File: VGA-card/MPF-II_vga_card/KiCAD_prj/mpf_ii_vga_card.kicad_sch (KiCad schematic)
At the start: 5 parts, among them J1 AppleBus, U1 74LVC245, U2 74LVC245, U3 74LVC245, U4 74LVC245

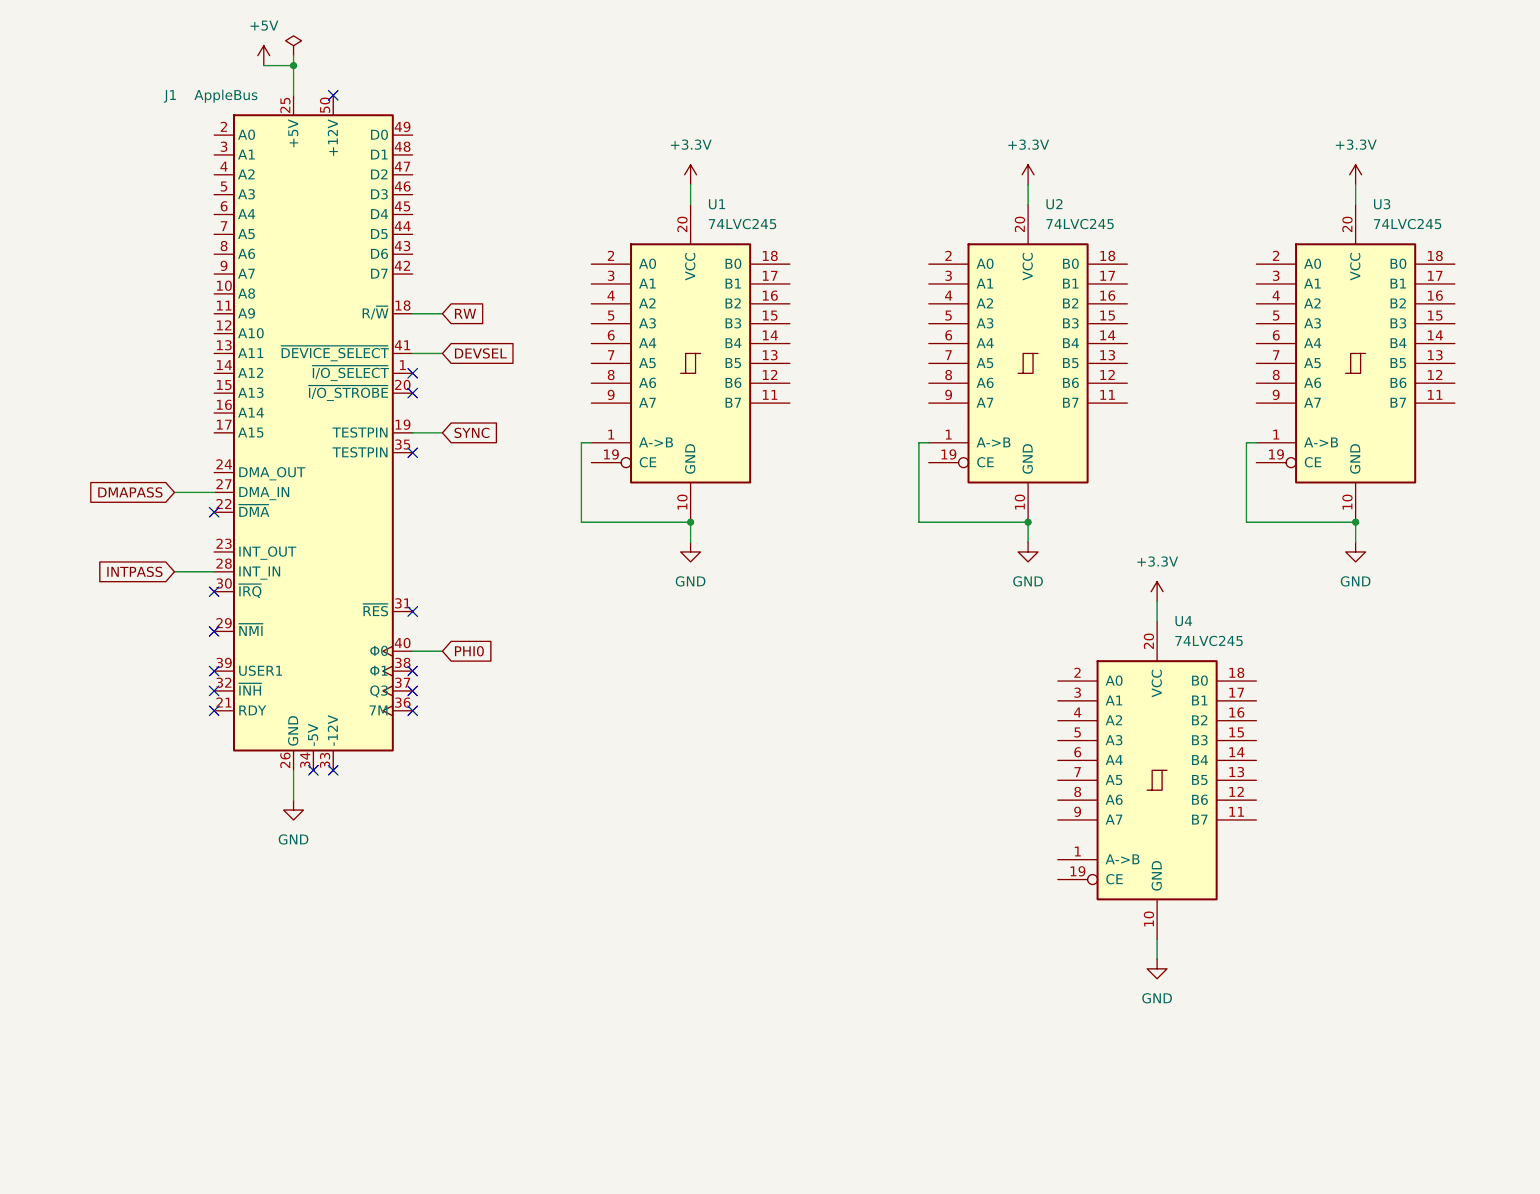
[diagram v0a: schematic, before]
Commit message: Schematics updated
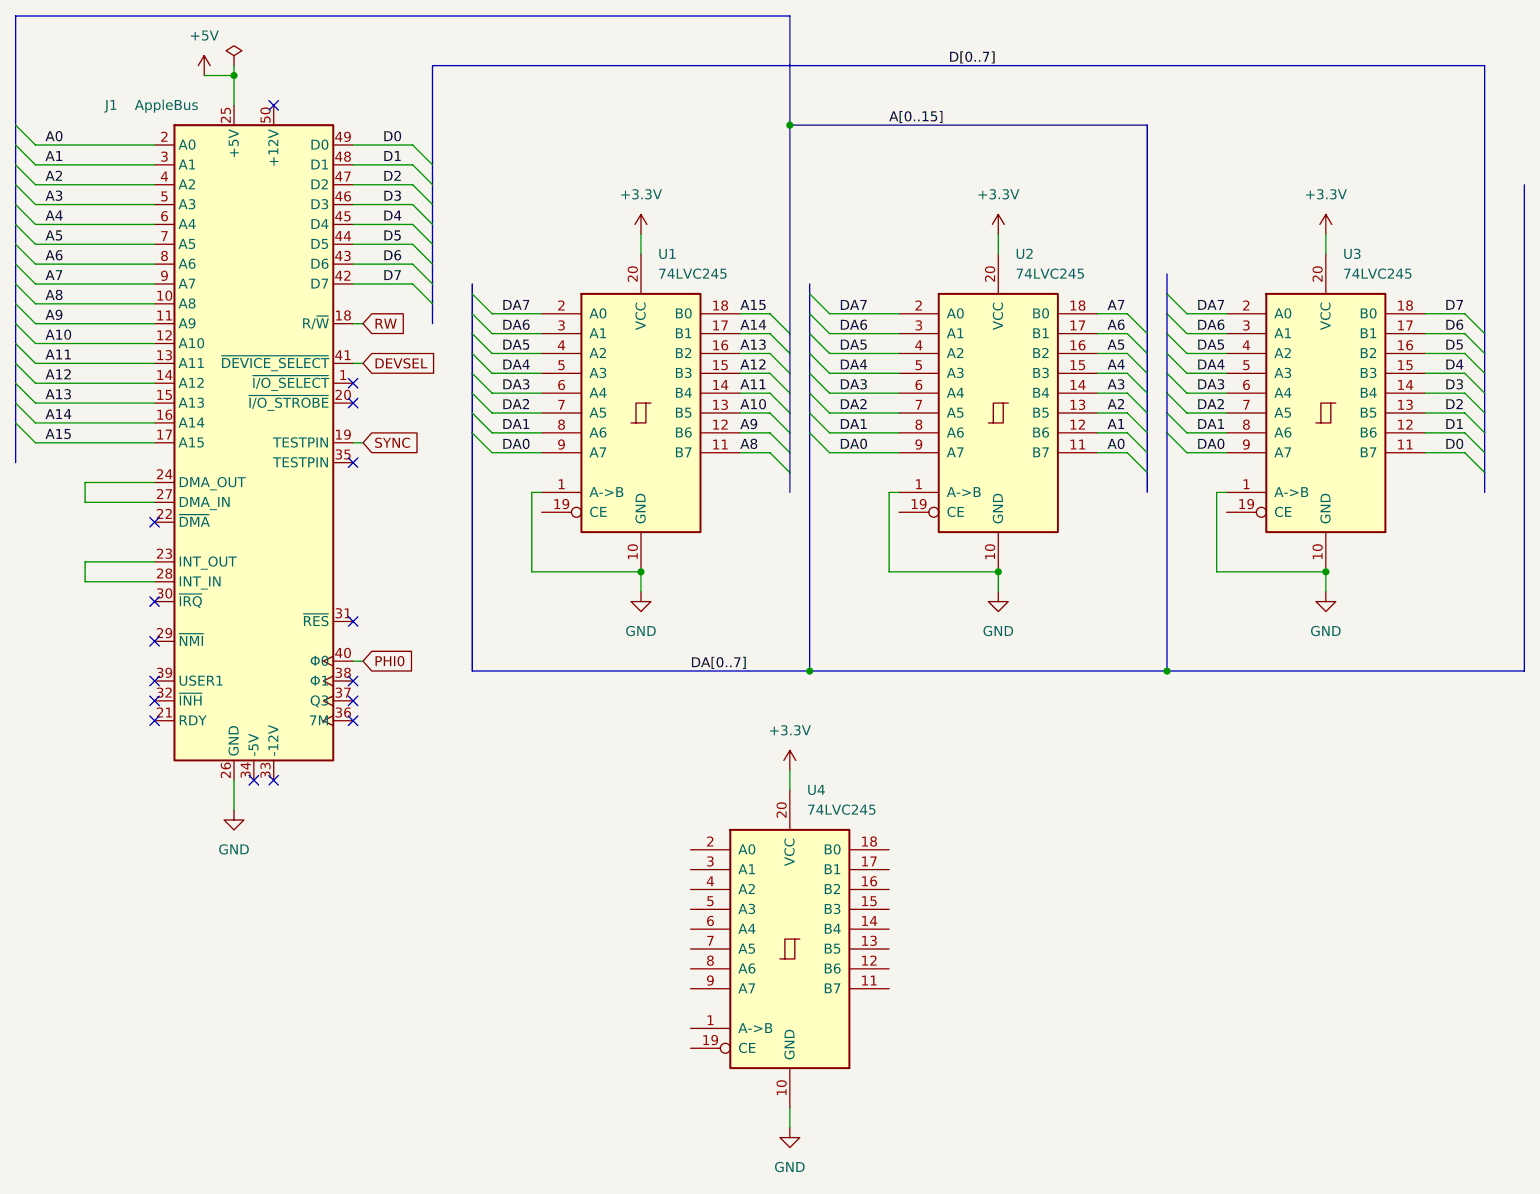
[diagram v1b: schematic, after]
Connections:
- net DMAPASS is gone; now on an unnamed net: J1.27 (DMA_IN)
- net INTPASS is gone; now on an unnamed net: J1.28 (INT_IN)
- net A8: now reaches J1.10 (A8)
- net A8: now also U1.11 (B7)
- net A9: now reaches J1.11 (A9)
- net A9: now also U1.12 (B6)
- net A10: now reaches J1.12 (A10)
- net A10: now also U1.13 (B5)
- net A11: now reaches J1.13 (A11)
- net A11: now also U1.14 (B4)
- net A12: now reaches J1.14 (A12)
- net A12: now also U1.15 (B3)
- net A13: now reaches J1.15 (A13)
- net A13: now also U1.16 (B2)
- net A14: now reaches J1.16 (A14)
- net A14: now also U1.17 (B1)
- net A15: now reaches J1.17 (A15)
- net A15: now also U1.18 (B0)
- net A0: now reaches J1.2 (A0)
- net A0: now also U2.11 (B7)
- net A1: now reaches J1.3 (A1)
- net A1: now also U2.12 (B6)
- net A2: now reaches J1.4 (A2)
- net A2: now also U2.13 (B5)
- net D7: now reaches J1.42 (D7)
- net D7: now also U3.18 (B0)
- net D6: now reaches J1.43 (D6)
- net D6: now also U3.17 (B1)
- net D5: now reaches J1.44 (D5)
- net D5: now also U3.16 (B2)
- net D4: now reaches J1.45 (D4)
- net D4: now also U3.15 (B3)
- net D3: now reaches J1.46 (D3)
- net D3: now also U3.14 (B4)
- net D2: now reaches J1.47 (D2)
- net D2: now also U3.13 (B5)
- net D1: now reaches J1.48 (D1)
- net D1: now also U3.12 (B6)
- net D0: now reaches J1.49 (D0)
- net D0: now also U3.11 (B7)
- net A3: now reaches J1.5 (A3)
- net A3: now also U2.14 (B4)
- net A4: now reaches J1.6 (A4)
- net A4: now also U2.15 (B3)
- net A5: now reaches J1.7 (A5)
- net A5: now also U2.16 (B2)
- net A6: now reaches J1.8 (A6)
- net A6: now also U2.17 (B1)
- net A7: now reaches J1.9 (A7)
- net A7: now also U2.18 (B0)
- net DA7: now reaches U3.2 (A0)
- net DA7: now also U1.2 (A0), U2.2 (A0)
- net DA6: now reaches U3.3 (A1)
- net DA6: now also U1.3 (A1), U2.3 (A1)
- net DA5: now reaches U3.4 (A2)
- net DA5: now also U1.4 (A2), U2.4 (A2)
- net DA4: now reaches U3.5 (A3)
- net DA4: now also U1.5 (A3), U2.5 (A3)
- net DA3: now reaches U3.6 (A4)
- net DA3: now also U1.6 (A4), U2.6 (A4)
- net DA2: now reaches U3.7 (A5)
- net DA2: now also U1.7 (A5), U2.7 (A5)
- net DA1: now reaches U3.8 (A6)
- net DA1: now also U1.8 (A6), U2.8 (A6)
- net DA0: now reaches U3.9 (A7)
- net DA0: now also U1.9 (A7), U2.9 (A7)
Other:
- moved on the sheet: J1, U1, U2, U3, U4
